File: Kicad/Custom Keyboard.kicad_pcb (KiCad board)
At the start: 2 copper layers, 349.3 x 133.3 mm, 216 parts, among them SW1 SW_Push, SW10 SW_Push, SW11 SW_Push, SW12 SW_Push, SW13 SW_Push, SW14 SW_Push, SW15 SW_Push, SW16 SW_Push, SW17 SW_Push, SW18 SW_Push, SW19 SW_Push, SW2 SW_Push, SW20 SW_Push, SW21 SW_Push, SW22 SW_Push, SW23 SW_Push, SW24 SW_Push, SW25 SW_Push, SW26 SW_Push, SW27 SW_Push, SW28 SW_Push, SW29 SW_Push, SW3 SW_Push, SW30 SW_Push, SW31 SW_Push, SW32 SW_Push, SW33 SW_Push, SW34 SW_Push, SW35 SW_Push, SW36 SW_Push, SW37 SW_Push, SW38 SW_Push, SW39 SW_Push, SW4 SW_Push, SW40 SW_Push, SW41 SW_Push, SW42 SW_Push, SW43 SW_Push, SW44 SW_Push, SW45 SW_Push, SW46 SW_Push, SW47 SW_Push, SW48 SW_Push, SW49 SW_Push, SW5 SW_Push, SW50 SW_Push, SW51 SW_Push, SW52 SW_Push, SW53 SW_Push, SW54 SW_Push, SW55 SW_Push, SW56 SW_Push, SW57 SW_Push, SW58 SW_Push, SW59 SW_Push, SW6 SW_Push, SW60 SW_Push, SW61 SW_Push, SW62 SW_Push, SW63 SW_Push, SW64 SW_Push, SW65 SW_Push, SW66 SW_Push, SW7 SW_Push, SW8 SW_Push, SW9 SW_Push, U1 ER_OLEDM0.91_1x-I2C, U4 PCF8574AP

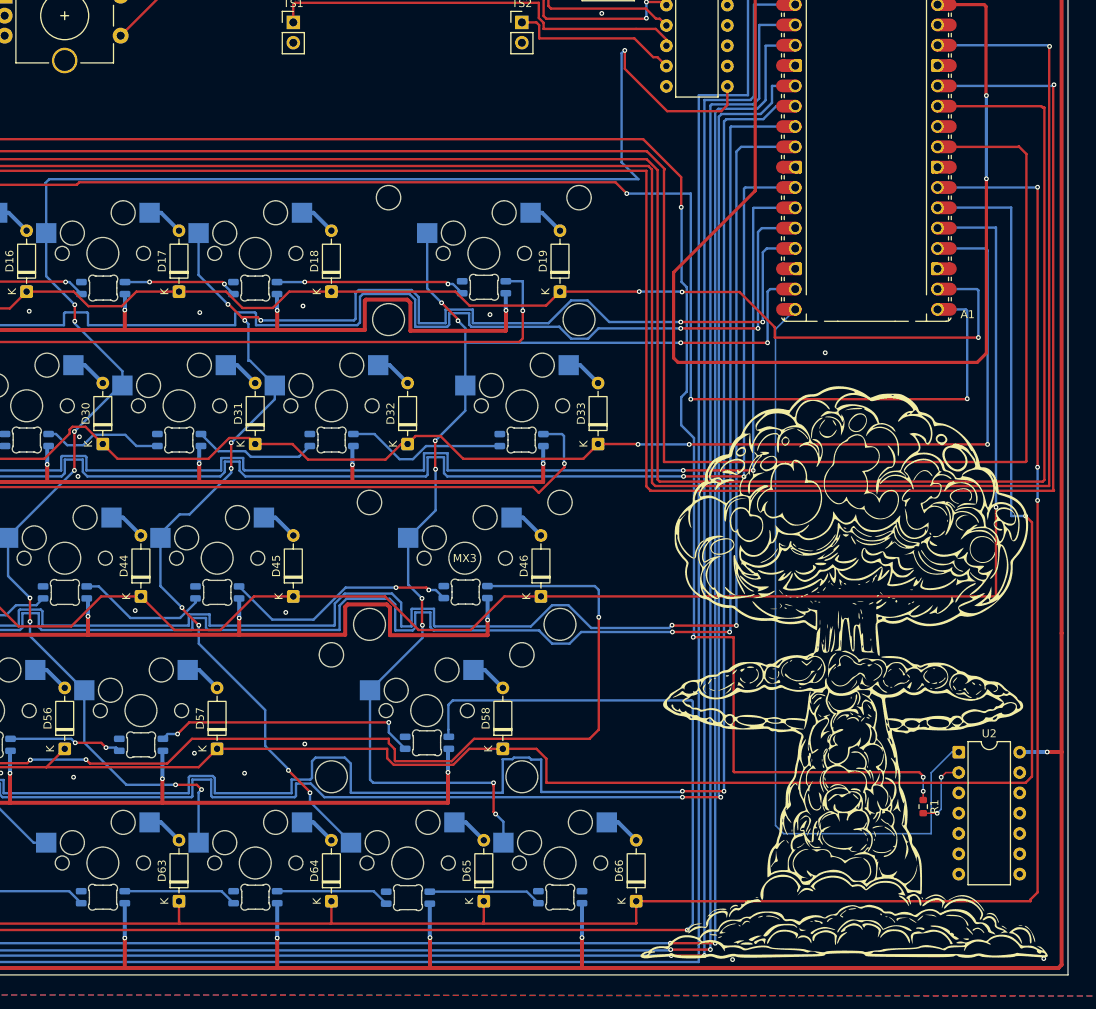
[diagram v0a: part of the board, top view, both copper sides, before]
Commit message: reolacing files
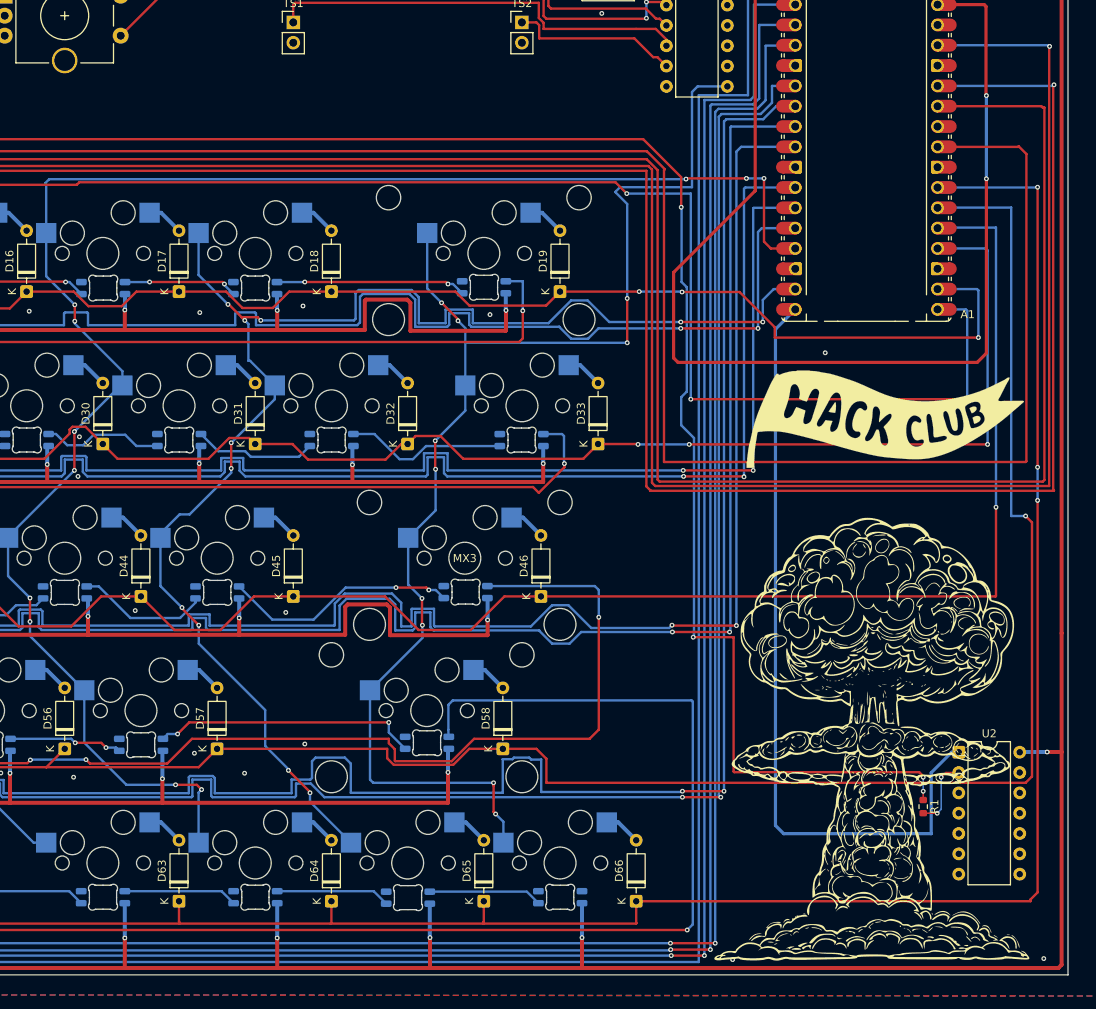
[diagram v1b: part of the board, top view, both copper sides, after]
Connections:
- A1 pad 17: /C12 -> /C11
- A1 pad 19: /C13 -> /C12
- U2 pad : (no net) -> Net-(RGB_LED1-DIN)
- U2 pad 1: (no net) -> /RGB Data
- U4 pad 9: /C11 -> /C13
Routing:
- net /C13: track 148.1 -> 166.5 mm
- net /C11: track 219.3 -> 209.3 mm, vias 9 -> 11
- net /C12: track 187.9 -> 182.3 mm
